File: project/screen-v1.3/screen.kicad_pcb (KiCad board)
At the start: 4 copper layers, 41.9 x 30 mm, 37 parts, among them J1 TTL-connect-pin4, J2 USB_C_6pin, J3 Conn_01x02_Female, Q1 S8050, SW1 SW_DPDT_x2, SW2 SW_Push, SW3 SW_Push, U1 SPX3819M5-L-3-3, U2 ESP-12E, U3 TFT_1.3_12, U4 TP4056_[C16581]

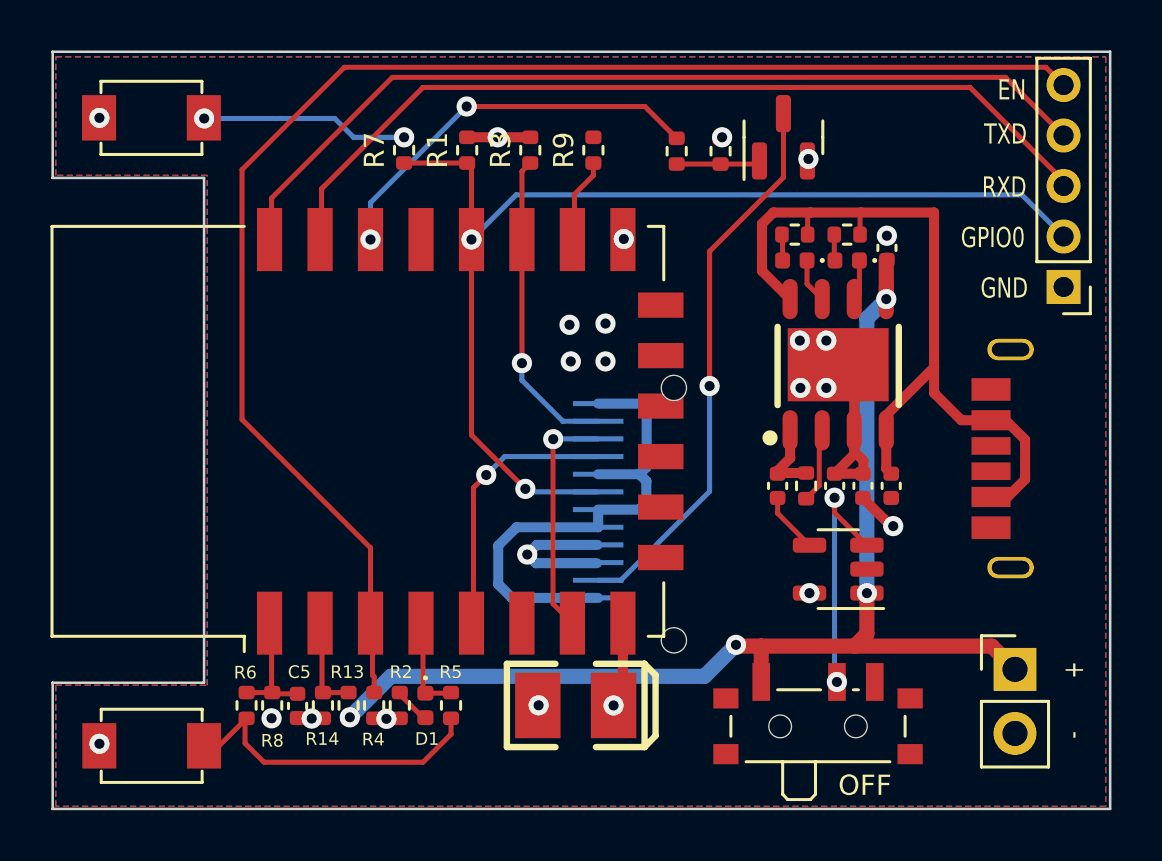
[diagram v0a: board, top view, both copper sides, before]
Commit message: update
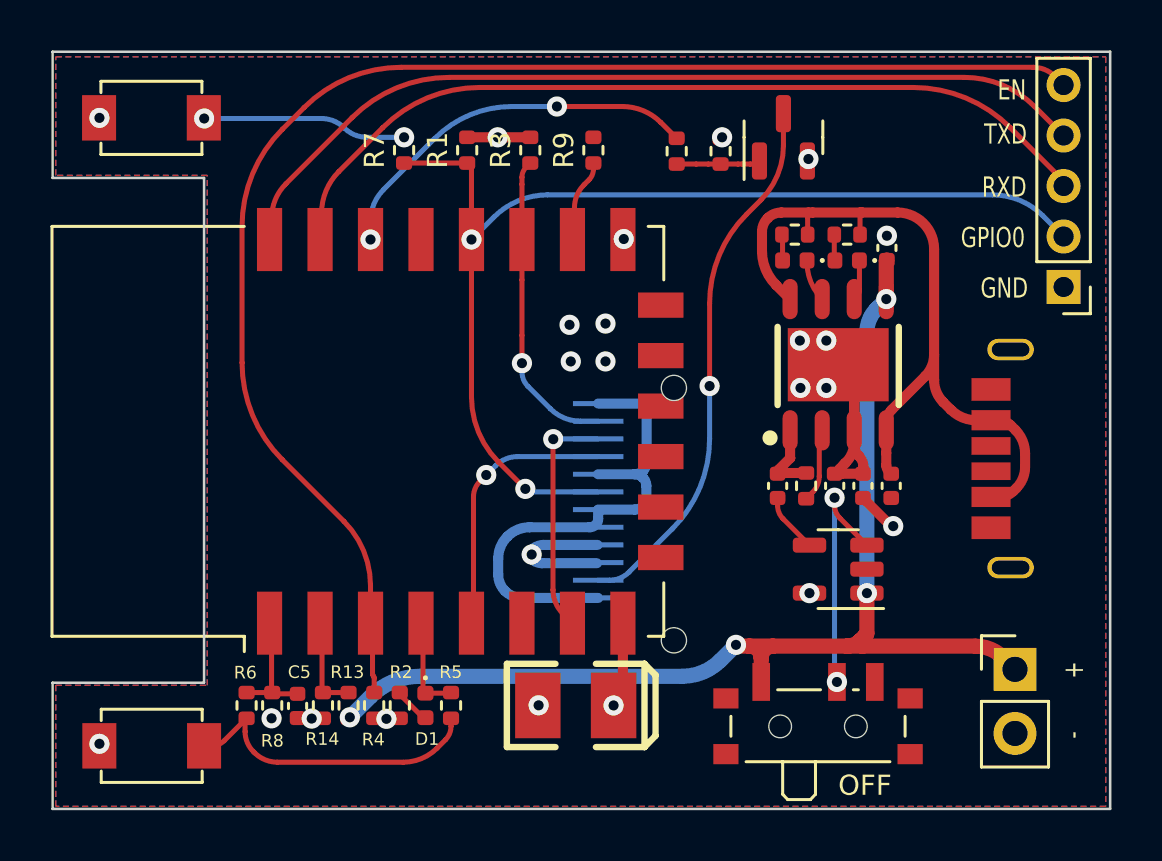
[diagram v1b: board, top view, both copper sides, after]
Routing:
- net +BATT: track 45.3 -> 46.4 mm
- net /EN: track 57.4 -> 56.4 mm
- net Net-(Q1-Pad3): track 22.1 -> 21.4 mm
- net /RXD: track 34.7 -> 34.1 mm
- net /TXD: track 35.9 -> 35.4 mm
